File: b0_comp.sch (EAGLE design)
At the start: 255 parts, among them IC1 КР1006ВИ1(NE555), IC3 LM358D, IC4 78L09F, IC6 MEGA8-AI, IC7 74121N, IC8 4030N, IC9 LM324D, T1P T, T1P1 T

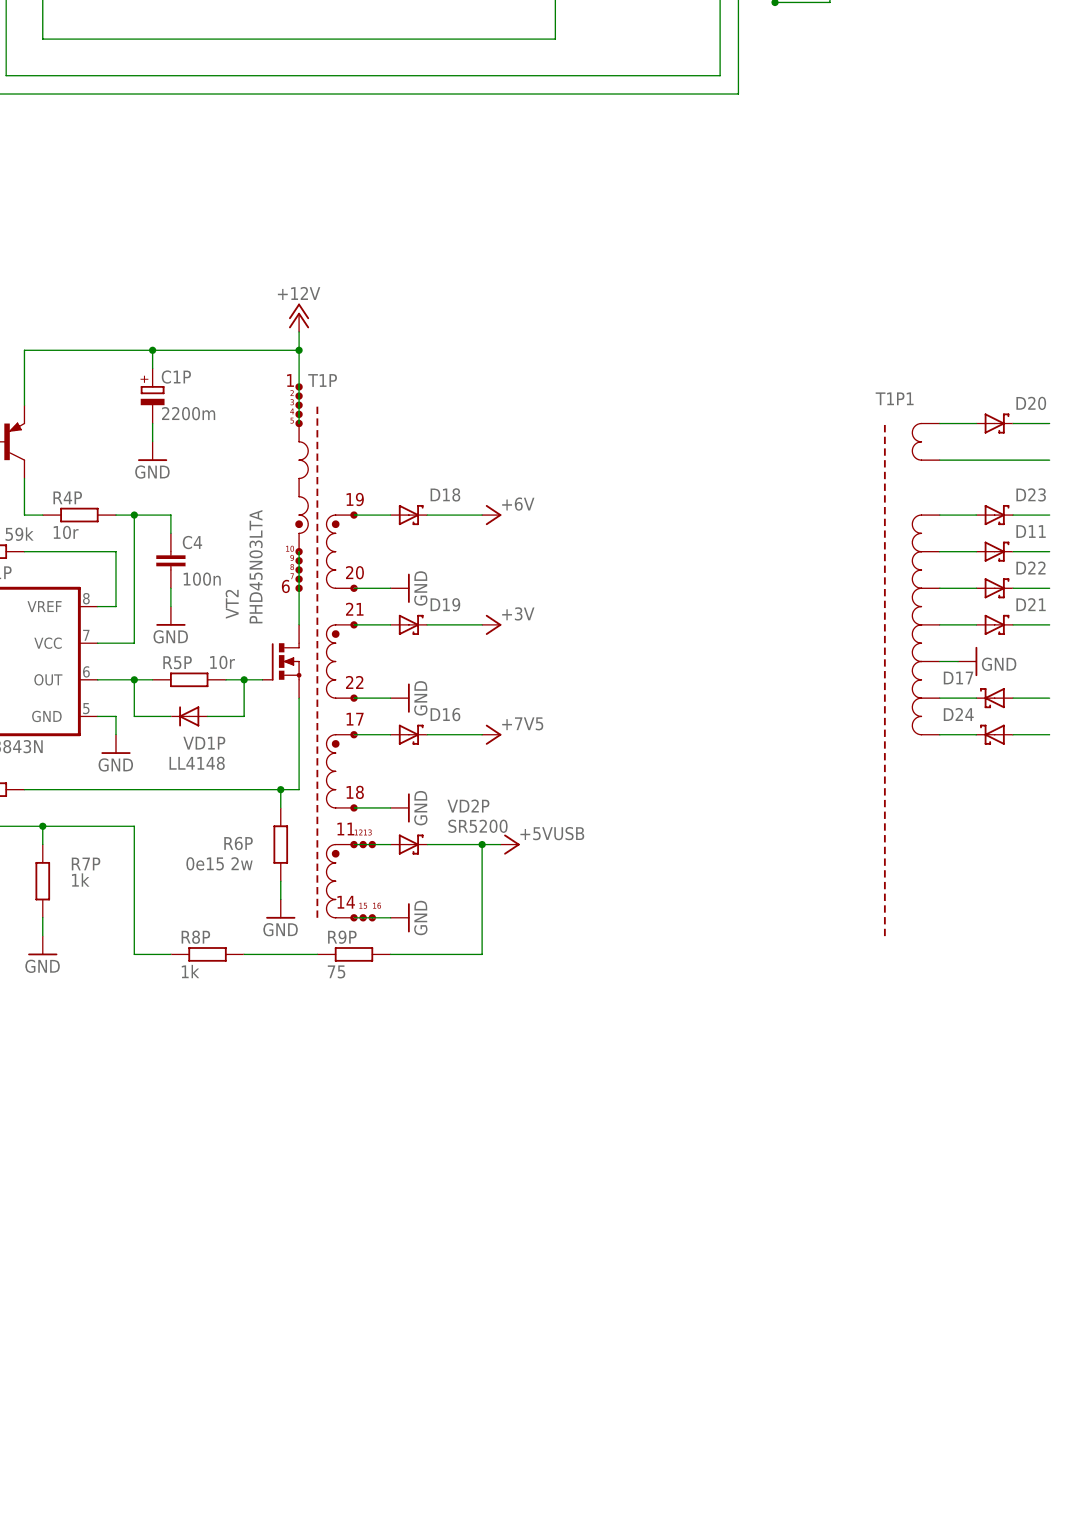
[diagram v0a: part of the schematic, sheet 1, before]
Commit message: .
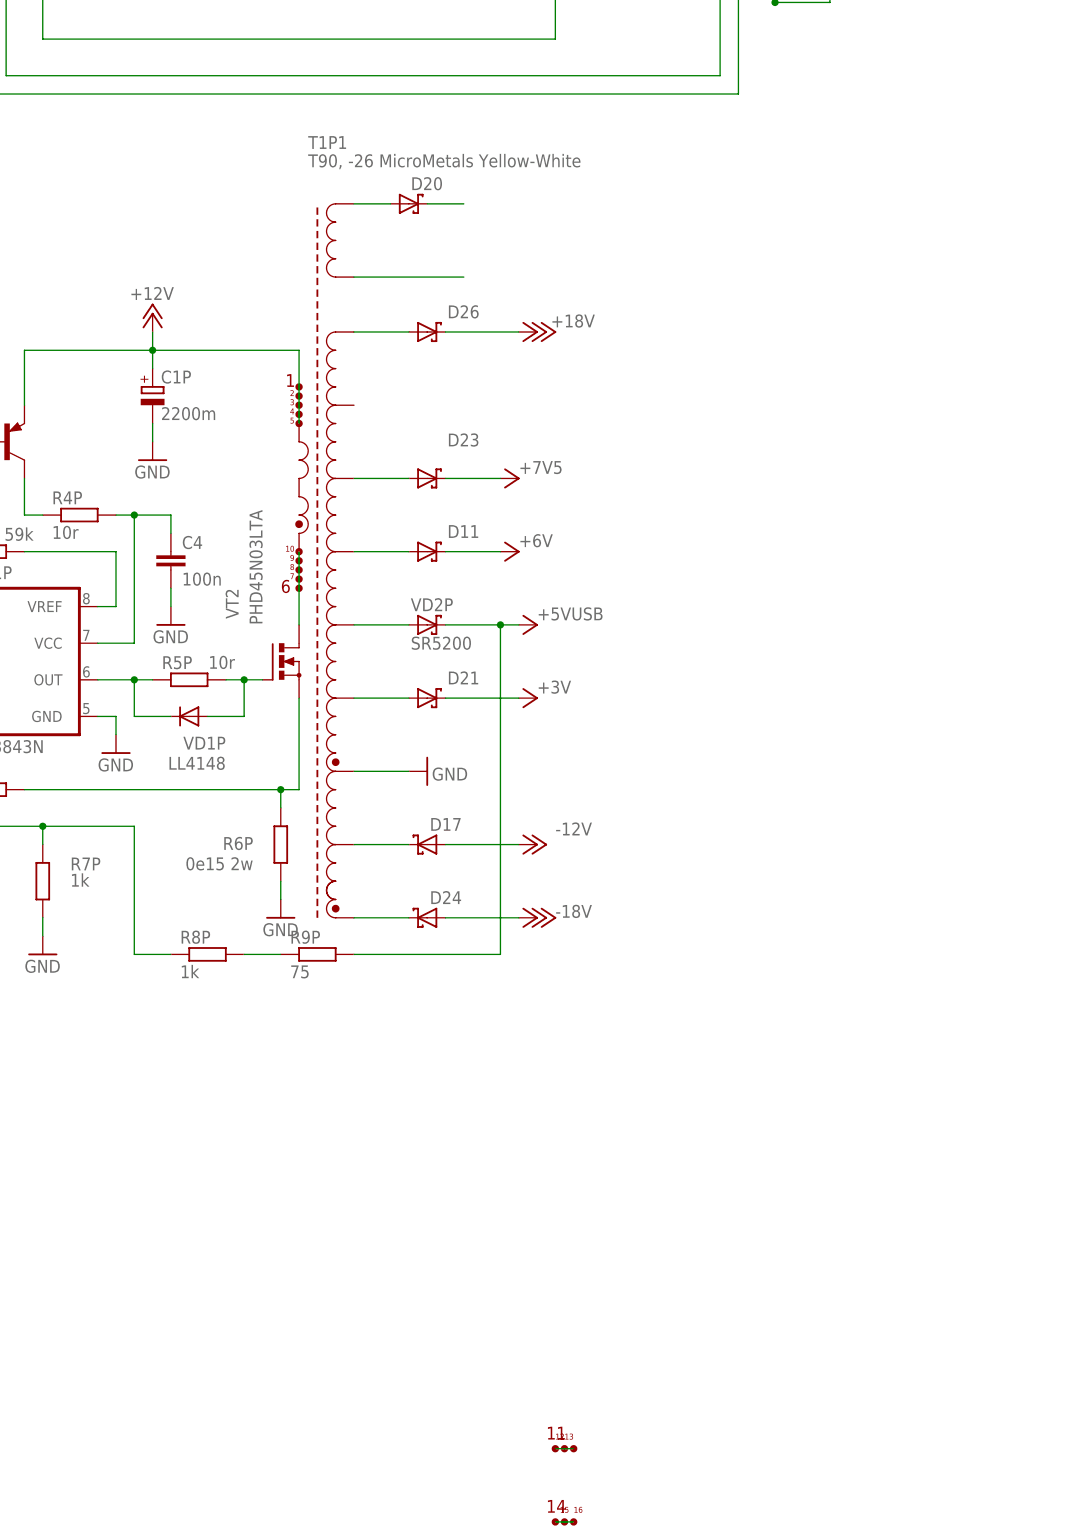
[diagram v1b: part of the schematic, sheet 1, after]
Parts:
- removed 17, 18, 19, 20, 21, 22: T_PIN, b0f:T_PIN
- removed D16, D18, D19, D22: (no value), diode:SCHOTTKY-DIODECB429-17
- removed T1P: T, b0f:T
- added D26: (no value), diode:SCHOTTKY-DIODECB429-17
- T1P1: value T -> T90, -26 MicroMetals Yellow-White
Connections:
- net N$179 renamed -18V
- removed net N$107: 19.P$1, D18.A
- removed net N$162: 21.P$1, D19.A
- removed net N$169: D21.C
- removed net N$170: D11.C
- removed net N$174: D22.C
- removed net N$176: D23.C
- removed net N$177: D17.A
- new net +18V: D26.C
- new net N$180: D26.A
- net +3V: now also D21.C; no longer D19.C
- net +6V: now also D11.C; no longer D18.C
- net +7V5: now also D23.C; no longer D16.C
- net -12V: now also D17.A
- net GND: no longer 14.P$1, 15.P$1, 16.P$1, 18.P$1, 20.P$1, 22.P$1
- net N$173: now also VD2P.A; no longer D22.A
- net N$64: no longer VD2P.A
- net N$67: now also 14.P$1, 15.P$1, 16.P$1; no longer 17.P$1, D16.A
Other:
- note added: "10(0.3x1)"
- note added: "12v"
- note added: "14(0.3x1)"
- note added: "27"
- note added: "3(0.6x1)"
- note added: "30(0.3x1)"
- note added: "4(0.6x1)"
- note added: "5(0.6x4)"
- note added: "8(0.6x4)"
- note added: "T90, -26 MicroMetals Yellow-White"
- note removed: "-12vuart"
- note removed: "-15vuart"
- note removed: "3v"
- note removed: "5.1v2.4a 10w 0.6mm x3"
- note removed: "5vusb"
- note removed: "6v"
- note removed: "7.5v0.5a 15w 0.6mm x1"
- note removed: "7.6v"
- moved on the sheet: 11, 12, 13, 14, 15, 16, D11, D17, D20, D21, D23, D24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

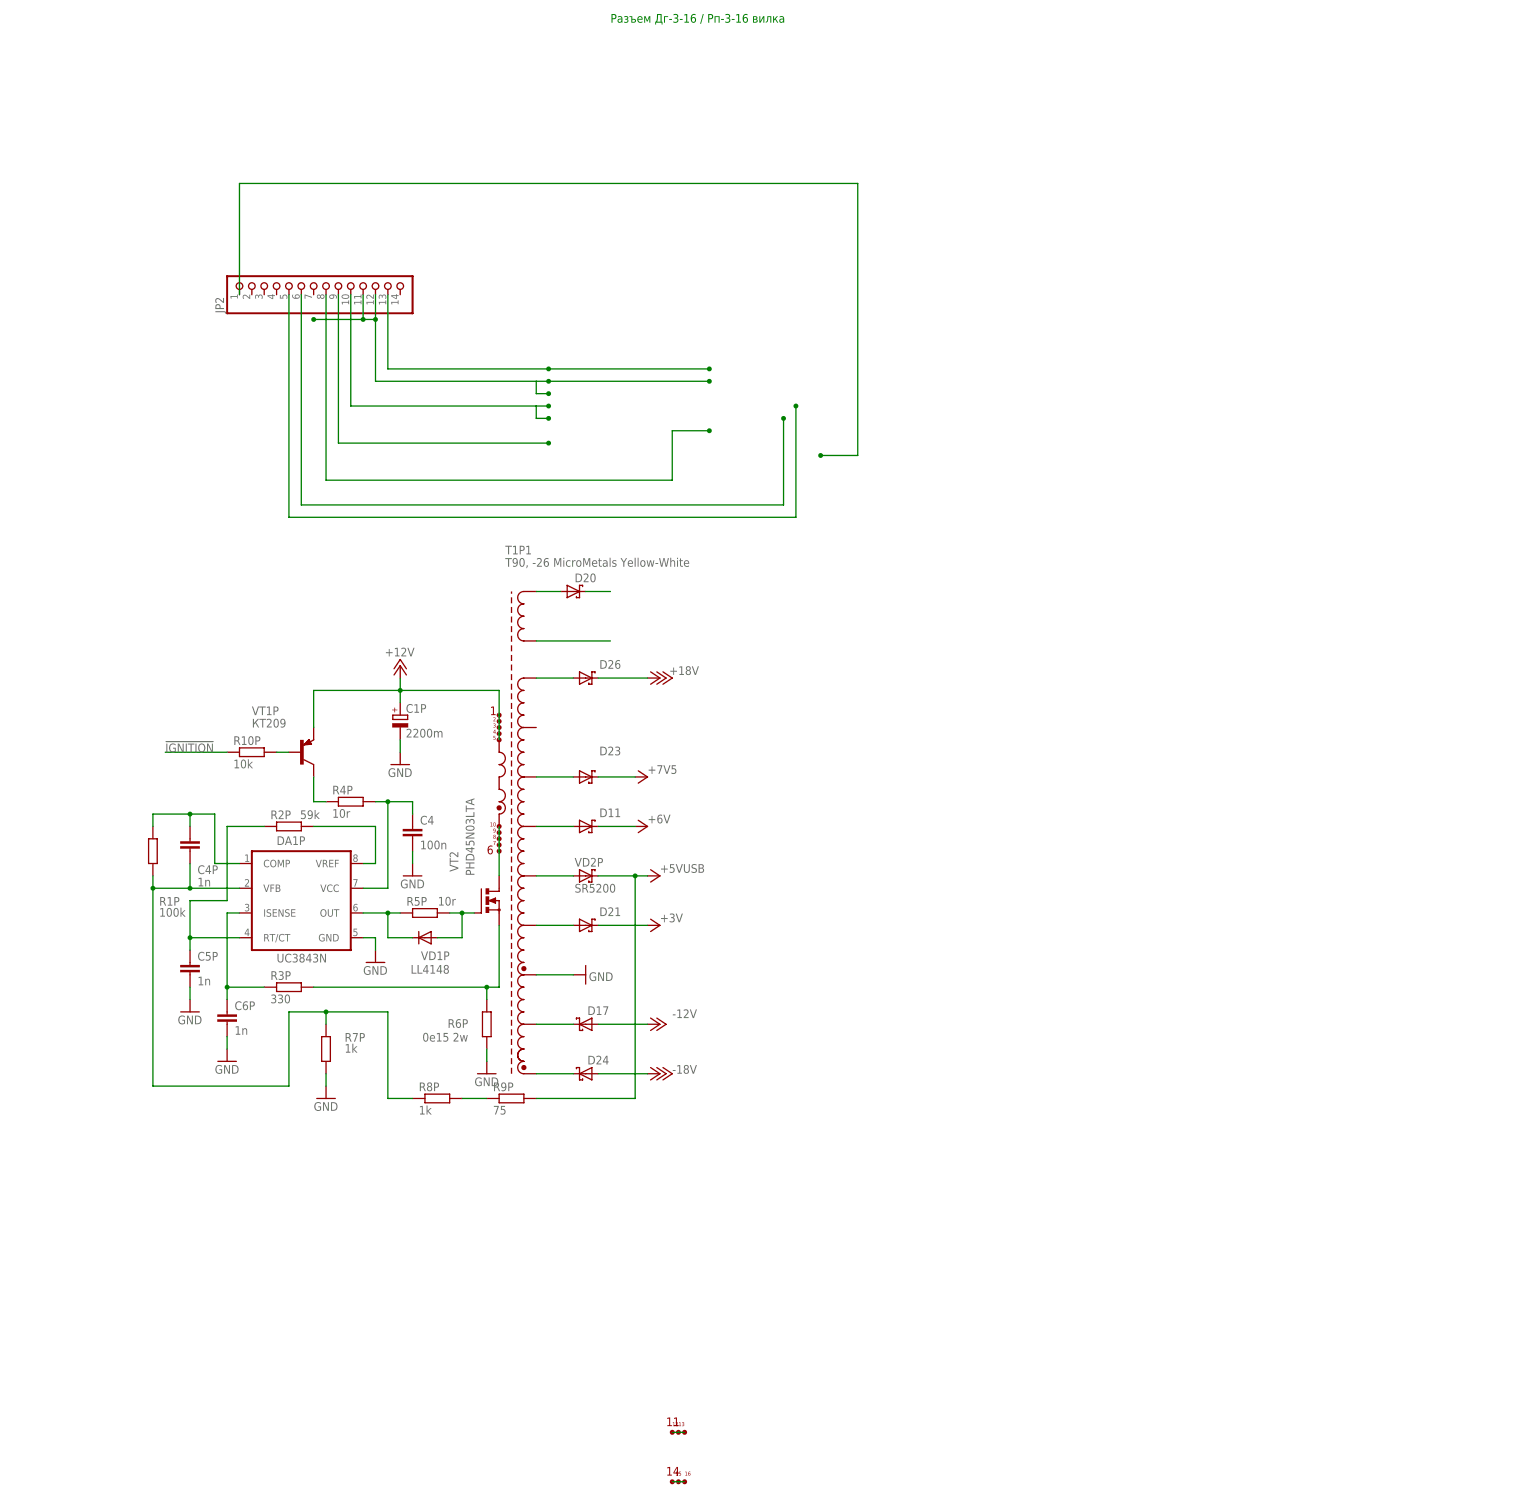
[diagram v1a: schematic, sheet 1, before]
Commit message: ..
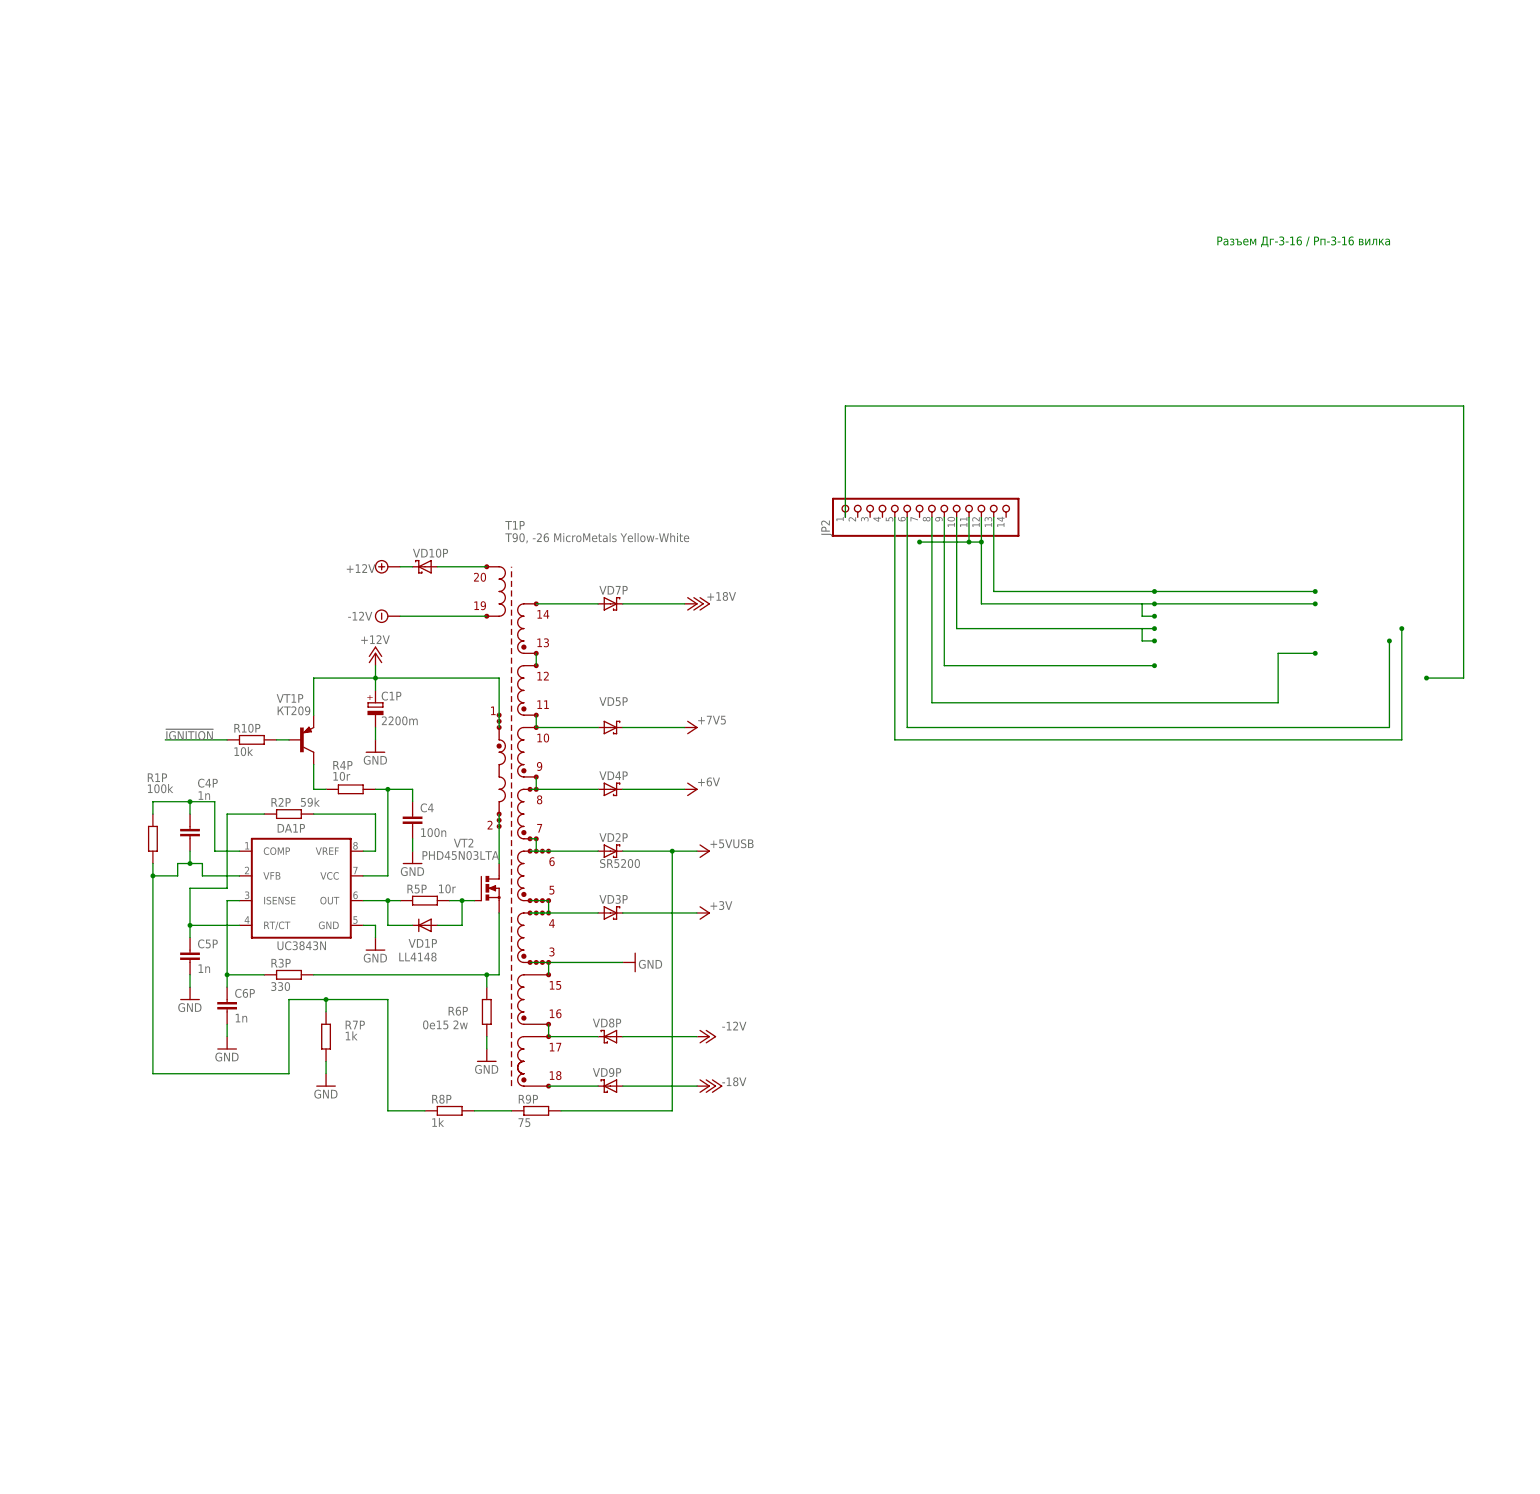
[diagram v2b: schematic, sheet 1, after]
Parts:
- removed D11, D17, D20, D21, D23, D24, D26: (no value), diode:SCHOTTKY-DIODECB429-17
- removed T1P1: T90, -26 MicroMetals Yellow-White, b0f:T
- added 17, 18, 19, 20: T_PIN, b0f:T_PIN
- added T1P: T90, -26 MicroMetals Yellow-White, b0f:T
- added U$19, U$20, U$21, U$22, U$23, U$24, U$25, U$26, U$27, U$28, U$29, U$30, U$31, U$32, U$33, U$34, U$35, U$36: T_PIN_NONAME, b0f:T_PIN_NONAME
- added VD10P, VD3P, VD4P, VD5P, VD7P, VD8P, VD9P: (no value), diode:SCHOTTKY-DIODECB429-17
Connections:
- removed net N$165: D21.A
- removed net N$166: D11.A
- removed net N$171: D20.C
- removed net N$173: VD2P.A
- new net N$107: 4.P$1, 5.P$1, U$26.TNN1, U$27.TNN1, U$28.TNN1, U$29.TNN1, U$30.TNN1, U$31.TNN1, VD3P.A
- new net N$162: 6.P$1, 7.P$1, U$32.TNN1, U$33.TNN1, U$34.TNN1, U$36.TNN1, VD2P.A
- net +12V: now also U$22.TNN1, U$23.TNN1, VD10P.C; no longer 2.P$1, 3.P$1, 4.P$1, 5.P$1
- net +18V: now also VD7P.C; no longer D26.C
- net +3V: now also VD3P.C; no longer D21.C
- net +6V: now also VD4P.C; no longer D11.C
- net +7V5: now also VD5P.C; no longer D23.C
- net -12V: now also 19.P$1, VD8P.A; no longer D17.A
- net -18V: now also VD9P.A; no longer D24.A
- net GND: now also 15.P$1, 3.P$1, U$19.TNN1, U$20.TNN1, U$21.TNN1
- net N$168: now also 20.P$1, VD10P.A; no longer D20.A
- net N$172: now also 16.P$1, 17.P$1, VD8P.C; no longer D17.C
- net N$175: now also 10.P$1, 11.P$1, VD5P.A; no longer D23.A
- net N$178: now also 18.P$1, VD9P.C; no longer D24.C
- net N$180: now also 14.P$1, VD7P.A; no longer D26.A
- net N$24: now also 2.P$1, U$24.TNN1, U$25.TNN1; no longer 10.P$1, 6.P$1, 7.P$1, 8.P$1, 9.P$1
- net N$64: now also 8.P$1, 9.P$1, U$35.TNN1, VD4P.A; no longer 11.P$1, 12.P$1, 13.P$1
- net N$67: now also 12.P$1, 13.P$1; no longer 14.P$1, 15.P$1, 16.P$1
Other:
- note added: "3(0.6x2)"
- note added: "I 13+12w 0.6mm x3"
- note added: "Бел."
- note added: "Жёлт."
- note added: "Жёлт. 12V"
- note added: "Жёлт. с Син."
- note added: "Зел."
- note added: "Зел.с Син."
- note added: "Красн."
- note added: "Син."
- note removed: "12v"
- note removed: "12vt"
- note removed: "27"
- note removed: "3(0.6x1)"
- note removed: "I 12w 0.6mm x5"
- moved on the sheet: 10, 11, 12, 13, 14, 15, 16, 2, 3, 4, 5, 6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
